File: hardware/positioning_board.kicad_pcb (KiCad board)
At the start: 4 copper layers, 83 x 43 mm, 50 parts, among them J1 Conn_01x04, J2 Conn_01x05, J3 Conn_01x05, J4 4P4C, J5 USB_C_Receptacle_USB2.0_16P, Q1 MMBT3904, Q2 MMBT3904, SW1 SW_Push, SW2 SW_Push, U1 AMS1117-3.3, U2 ESP32-S3-WROOM-1, U3 LSM6DS3, U4 SN65HVD1782DR, U5 TPS563200, U6 CH340K

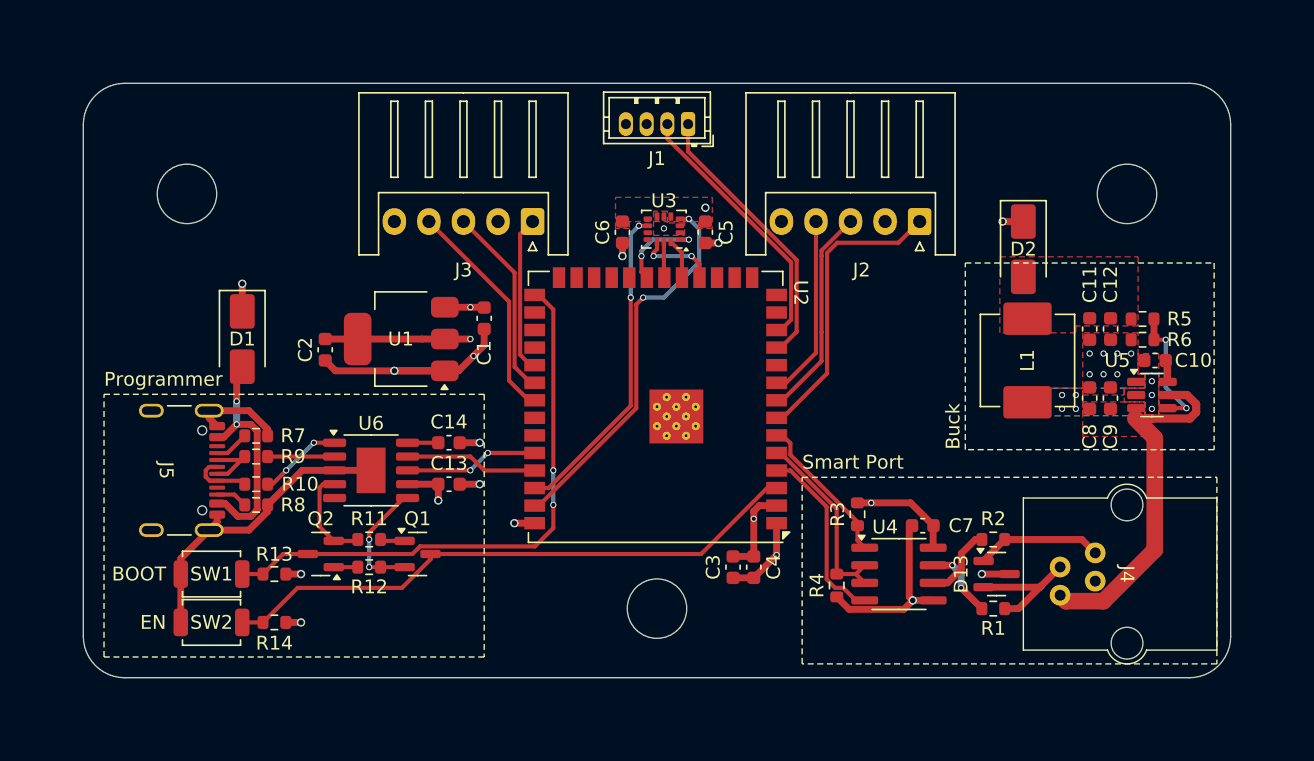
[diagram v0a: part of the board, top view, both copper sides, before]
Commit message: optimize size
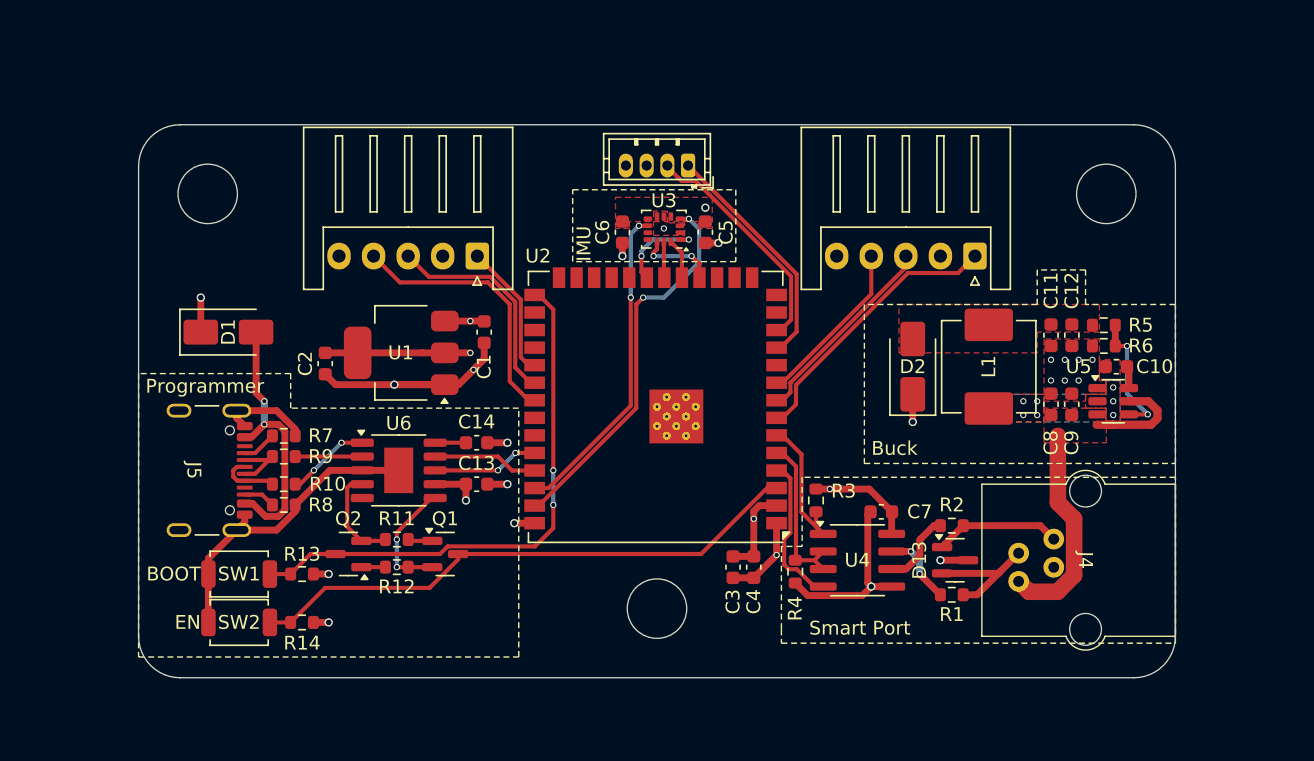
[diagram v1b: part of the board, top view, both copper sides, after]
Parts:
- moved D2 11.7 mm to (158.5, 87.5), turned to 90 degrees
- moved J2 4.72 mm to (163.0, 79.5)
- moved J3 4.72 mm to (127.0, 79.5)
- moved C7 3.16 mm to (156.2, 98.0)
- moved D13 3.16 mm to (161.6, 101.5)
- moved J4 3.16 mm to (171.0, 101.5)
- moved R1 3.16 mm to (161.3, 104.0)
- moved R2 3.16 mm to (161.3, 99.0)
- moved R3 3.16 mm to (151.5, 97.2)
- moved R4 3.16 mm to (150.0, 102.3)
- moved U4 3.16 mm to (154.5, 101.5)
- moved J1 3.00 mm to (142.2, 73.0)
- moved C10 2.83 mm to (173.2, 87.5)
- moved L1 2.83 mm to (164.0, 87.5)
- moved R5 2.83 mm to (172.3, 84.5)
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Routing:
- net /12V_Buck/+12V: track 26.5 -> 23.3 mm
- net /LIDAR_RX: track 20.2 -> 17.2 mm
- net /Encoder2_X: track 16.4 -> 19.2 mm
- net /usb_port/+5V: track 17.0 -> 19.6 mm
- net /Brain_TX: track 13.3 -> 11.1 mm
- net /Brain_Dir: track 13.9 -> 11.8 mm
- net /MCU_EN: track 42.9 -> 40.9 mm
- net /GPIO0: track 41.5 -> 39.5 mm
- net /Prog_TX: track 9.61 -> 7.61 mm
- net /Prog_RX: track 9.72 -> 7.72 mm
- net /LIDAR_PWM: track 19.2 -> 17.3 mm
- net /Encoder2_A: track 14.0 -> 15.7 mm
- net /Encoder2_B: track 11.4 -> 9.86 mm
- net /Encoder1_B: track 21.3 -> 20.0 mm
- net /Encoder1_X: track 13.2 -> 12.3 mm
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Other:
- board size 83 x 43 mm -> 75 x 40 mm
- board text added: "IMU"
